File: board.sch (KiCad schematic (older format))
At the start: 21 parts, among them J1 TEMPS, J2 OLED, J3 RELAY, J4 RELAY_EN, J5 USB_B_Micro, J6 CONN_PROG, SW1 SW_RESET, U1 ESP32-WROOM-32, U2 AMS1117-3.3

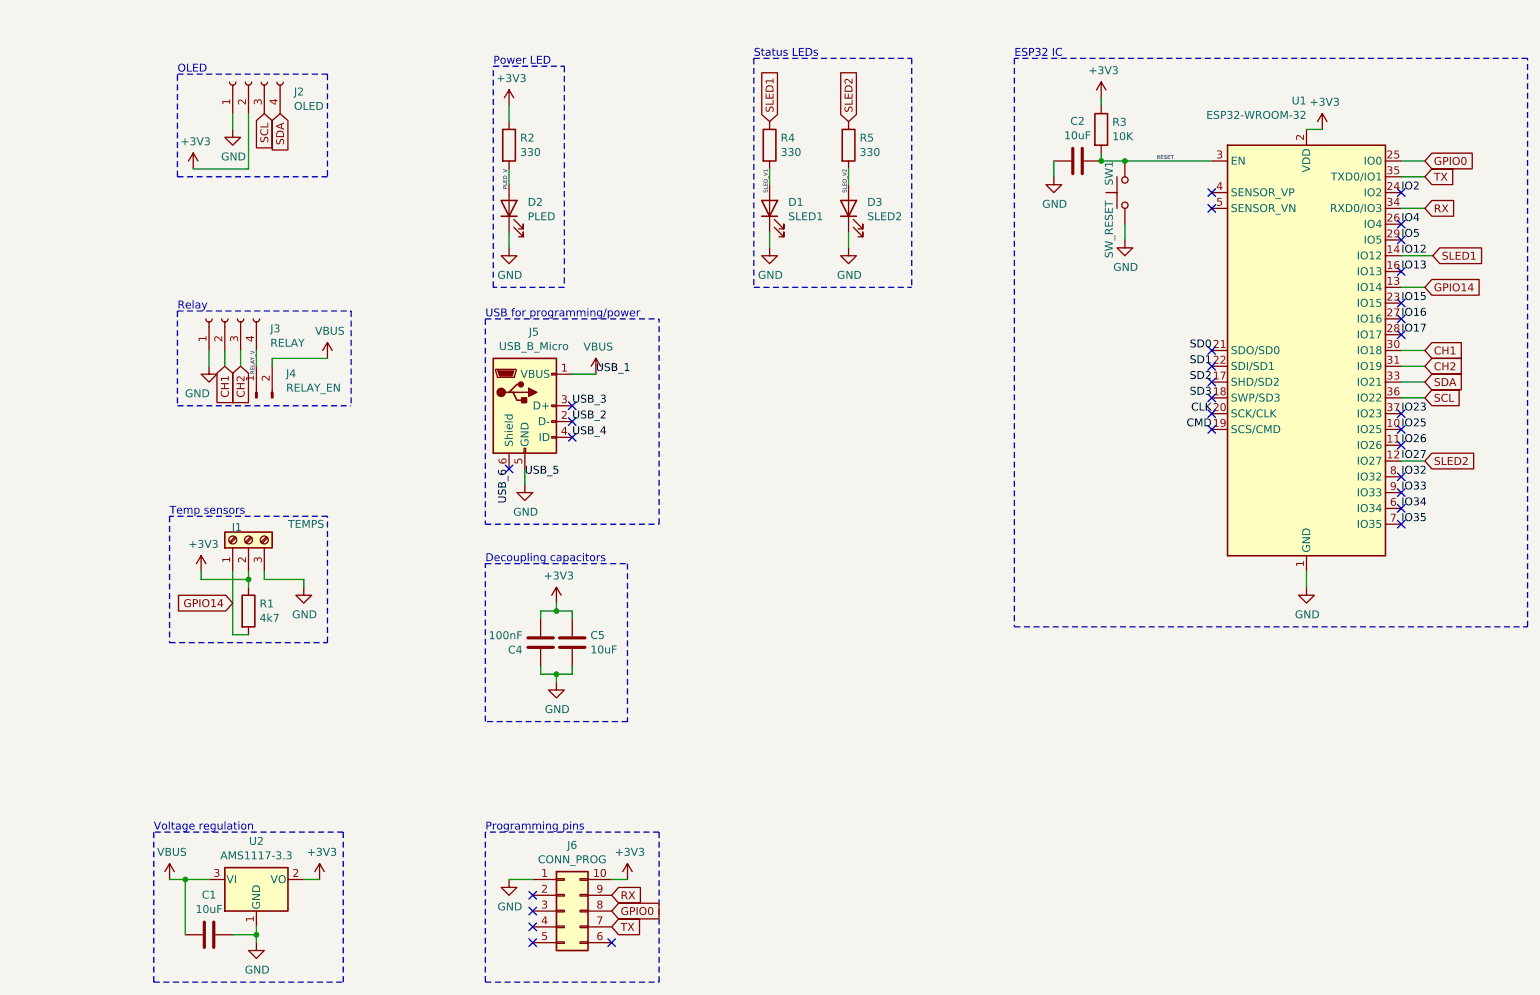
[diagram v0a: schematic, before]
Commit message: sourced components
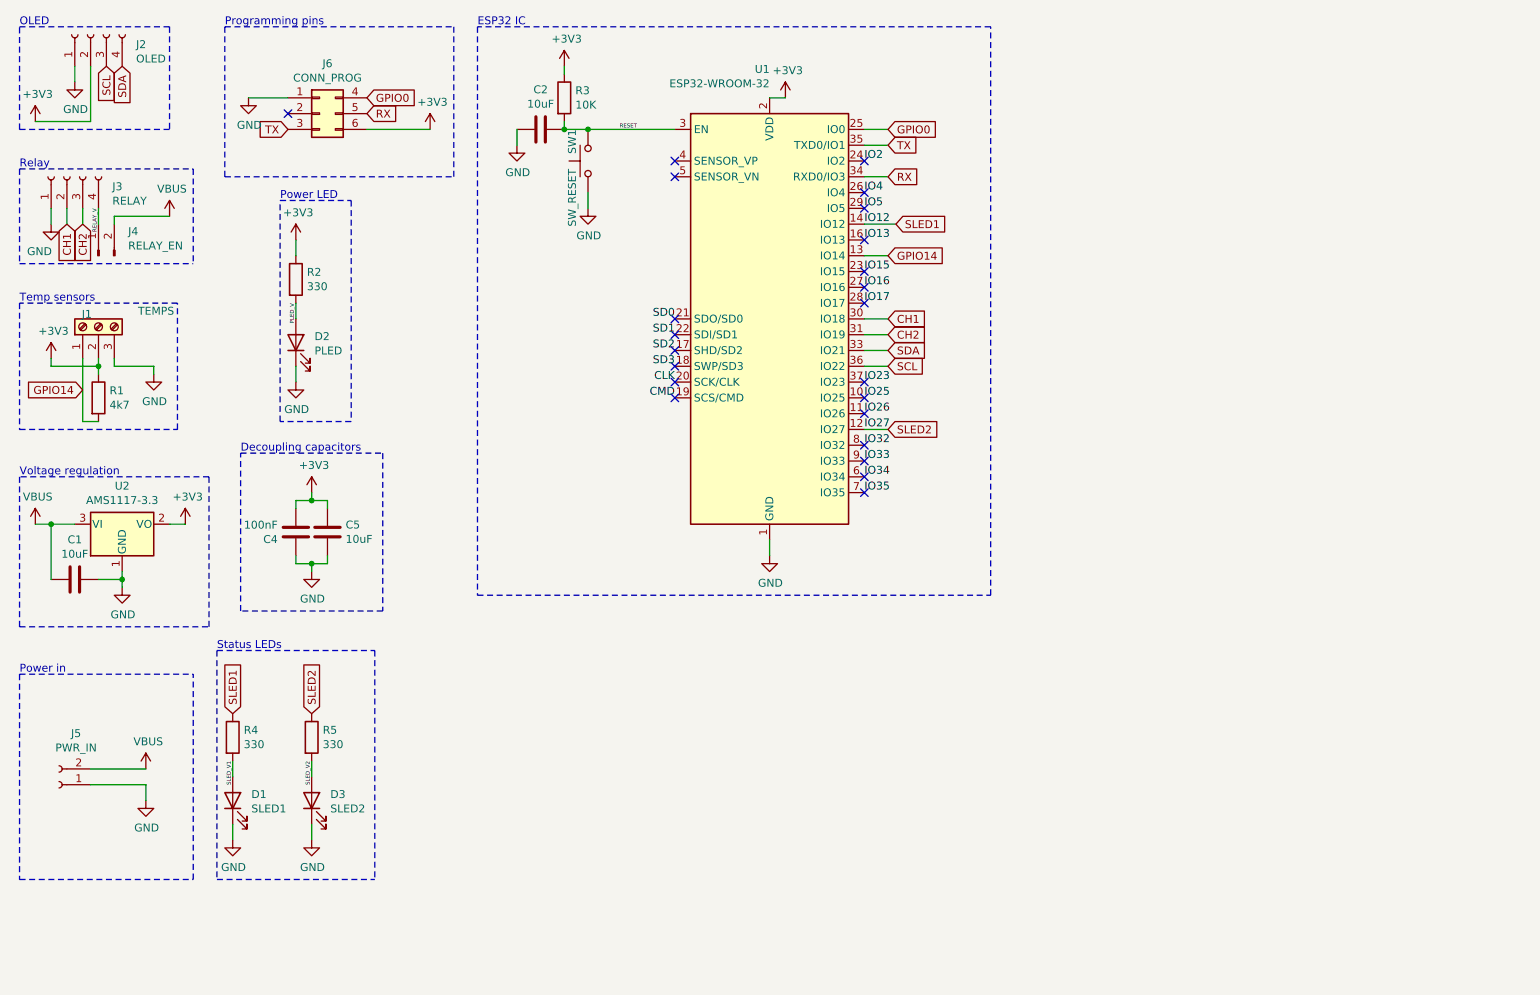
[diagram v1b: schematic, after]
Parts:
- removed J5: USB_B_Micro, Connector_USB:USB_Micro-B_Molex_47346-0001, symbol Connector:USB_B_Micro
- removed J6: CONN_PROG, Connector_PinHeader_1.27mm:PinHeader_2x05_P1.27mm_Vertical_SMD, symbol Connector_Generic:Conn_02x05_Counter_Clockwise
- added J5: PWR_IN, Connector_JST:JST_XH_S2B-XH-A-1_1x02_P2.50mm_Horizontal, symbol Connector:Conn_01x02_Female
- added J6: CONN_PROG, Connector_PinHeader_2.54mm:PinHeader_2x03_P2.54mm_Vertical, symbol Connector_Generic:Conn_02x03_Top_Bottom
- C1, C2, C5: Part No (none) -> C15850
- C4: Part No (none) -> C49678
- D1, D2, D3: footprint LED_SMD:LED_0805_2012Metric -> LED_SMD:LED_0603_1608Metric; Part No (none) -> C2286
- R1: Part No (none) -> C17673
- R2, R4, R5: Part No (none) -> C17630
- R3: Part No (none) -> C17414
- SW1: footprint Button_Switch_SMD:SW_SPST_B3U-1000P-B -> Button_Switch_THT:SW_PUSH_6mm_H13mm
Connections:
- net +3V3: now also J6.6 (Pin_6)
- net GND: now also J5.1 (Pin_1), J6.1 (Pin_1)
- net GPIO0: now also J6.4 (Pin_4)
- net RX: now also J6.5 (Pin_5)
- net TX: now also J6.3 (Pin_3)
- net VBUS: now also J5.2 (Pin_2)
- no-connect marks 31 -> 23
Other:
- note added: "Power in"
- note removed: "USB for programming/power"
- moved on the sheet: C1, C2, C4, C5, D1, D2, D3, J1, J2, J3, J4, R1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
